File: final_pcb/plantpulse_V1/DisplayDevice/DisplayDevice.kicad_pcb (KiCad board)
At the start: 2 copper layers, 119 x 64.2 mm, 10 parts, among them J1 SSD1306, M1 X27.168

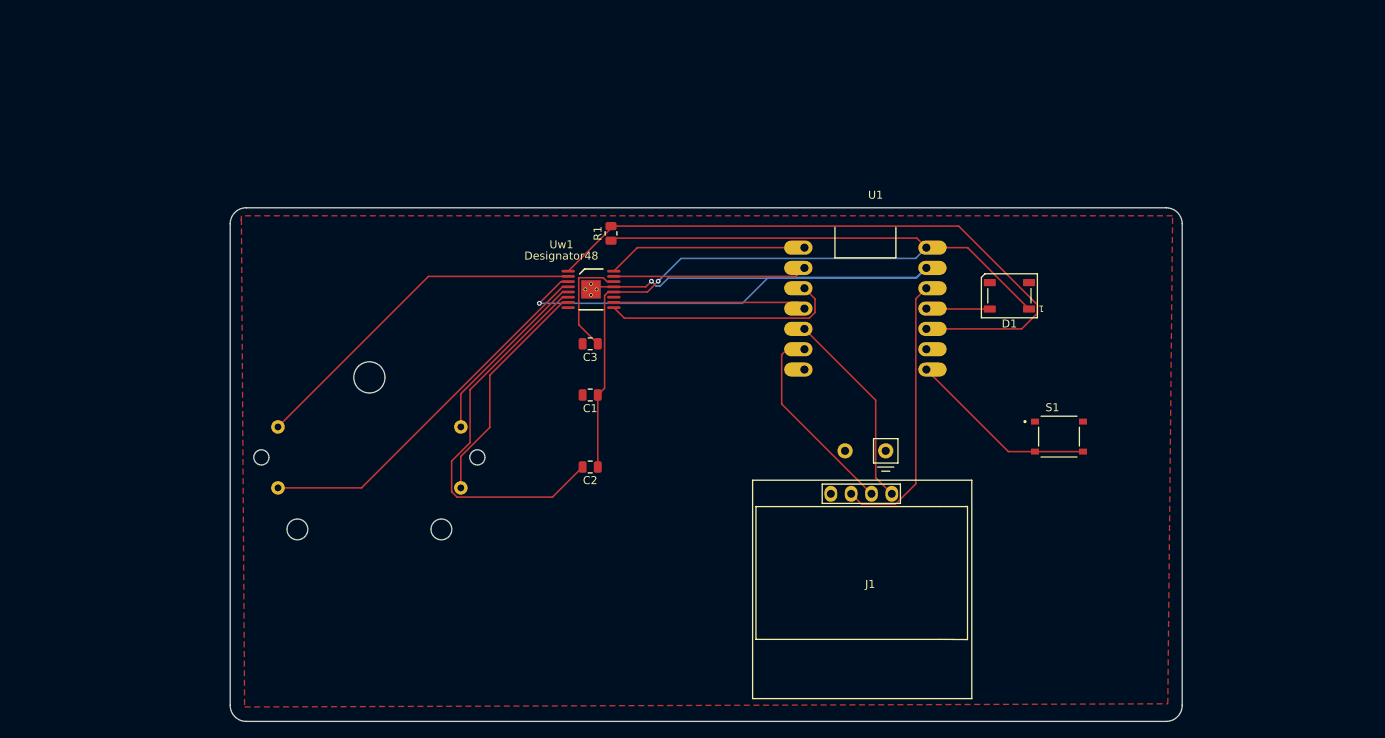
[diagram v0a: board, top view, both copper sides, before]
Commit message: Update
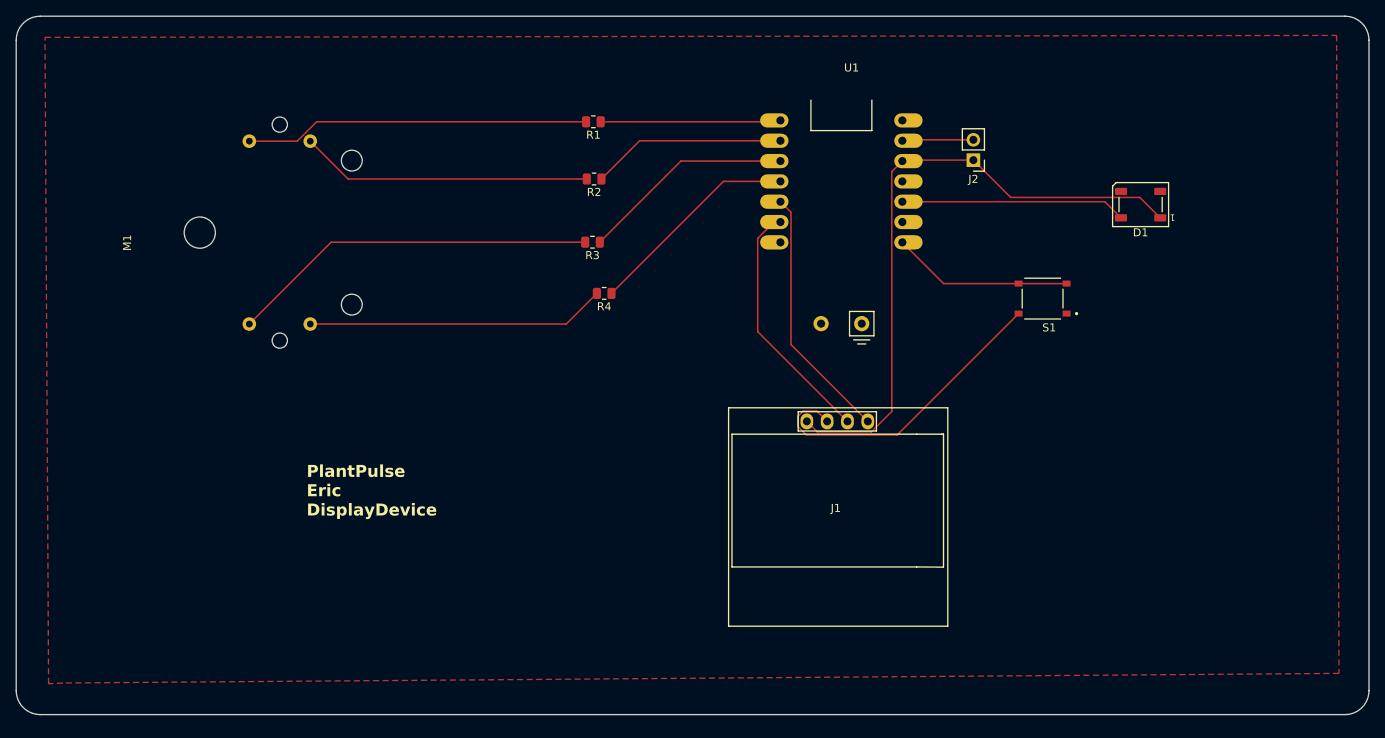
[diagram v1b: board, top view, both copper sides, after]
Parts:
- removed C1: 100nF, Capacitor_SMD:C_0805_2012Metric
- removed C2: 10uF, Capacitor_SMD:C_0805_2012Metric
- removed C3: 2.2uF, Capacitor_SMD:C_0805_2012Metric
- removed Uw1: DRV8833CPWPR, DRV8833:PWP0016K_N
- added J2: LiPo Battery, Connector_PinHeader_2.54mm:PinHeader_1x02_P2.54mm_Vertical, F.Cu at (179.7, 65.4)
- added R2: 47Ω, Resistor_SMD:R_0805_2012Metric, F.Cu at (132.3, 67.8)
- added R3: 47Ω, Resistor_SMD:R_0805_2012Metric, F.Cu at (132.1, 75.7)
- added R4: 47Ω, Resistor_SMD:R_0805_2012Metric, F.Cu at (133.6, 82.1)
- M1: moved to F.Cu
- R1: value 47kΩ -> 47Ω
- moved M1 40.8 mm to (103.2, 72.0), turned to 90 degrees
- moved D1 20.0 mm to (200.6, 71.0)
- moved S1 17.4 mm to (188.3, 82.8), turned to 180 degrees
- moved U1 16.2 mm to (163.2, 68.1)
- moved R1 14.1 mm to (132.2, 60.6), turned to 180 degrees
- moved J1 9.53 mm to (162.5, 108.7)
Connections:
- D1 pad 1: /5V -> /3V3
- J1 pad 1: /GND -> /3V3
- J1 pad 2: /3V3 -> /GND
- R1 pad 1: /5V -> Net-(U1-GPIO1_A0_D0)
- R1 pad 2: Net-(U1-GPIO8_A9_D9_CIPO) -> Net-(M1-Pin_1)
- U1 pad 10: Net-(U1-GPIO8_A9_D9_CIPO) -> Net-(D1-DIN)
- U1 pad 11: Net-(D1-DIN) -> unconnected-(U1-GPIO9_A10_D10_COPI-Pad11)
- U1 pad 14: /5V -> unconnected-(U1-5V-Pad14)
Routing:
- net /5V: track 120.5 -> 0.00 mm, vias 1 -> 0
- net /GND: track 148.8 -> 49.0 mm, vias 2 -> 0
- net Net-(U1-GPIO8_A9_D9_CIPO): track 81.0 -> 0.00 mm
- net /3V3: track 34.7 -> 79.3 mm
- net Net-(M1-Pin_3): track 22.8 -> 46.2 mm
- net Net-(D1-DIN): track 7.95 -> 28.2 mm
- net Net-(Uw1-VINT): track 13.8 -> 0.00 mm
- net Net-(M1-Pin_2): track 46.7 -> 36.5 mm
- net Net-(M1-Pin_4): track 29.2 -> 37.4 mm
- net Net-(J1-SDA): track 25.1 -> 32.0 mm
- net Net-(J1-SCL): track 25.2 -> 31.2 mm
- net Net-(U1-GPIO3_A2_D2): track 29.6 -> 26.8 mm
- net Net-(U1-GPIO4_A3_D3): track 24.2 -> 26.9 mm
- net Net-(U1-GPIO1_A0_D0): track 25.0 -> 22.5 mm
- net Net-(U1-GPIO44_D7_RX): track 23.8 -> 22.7 mm
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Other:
- board size 119 x 64.2 mm -> 169.1 x 87.3 mm
- board text added: "PlantPulse Eric DisplayDevice"
